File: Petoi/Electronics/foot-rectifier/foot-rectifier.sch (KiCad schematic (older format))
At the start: 6 parts, among them J1 Conn_01x04_Male, J2 Conn_01x02_Male

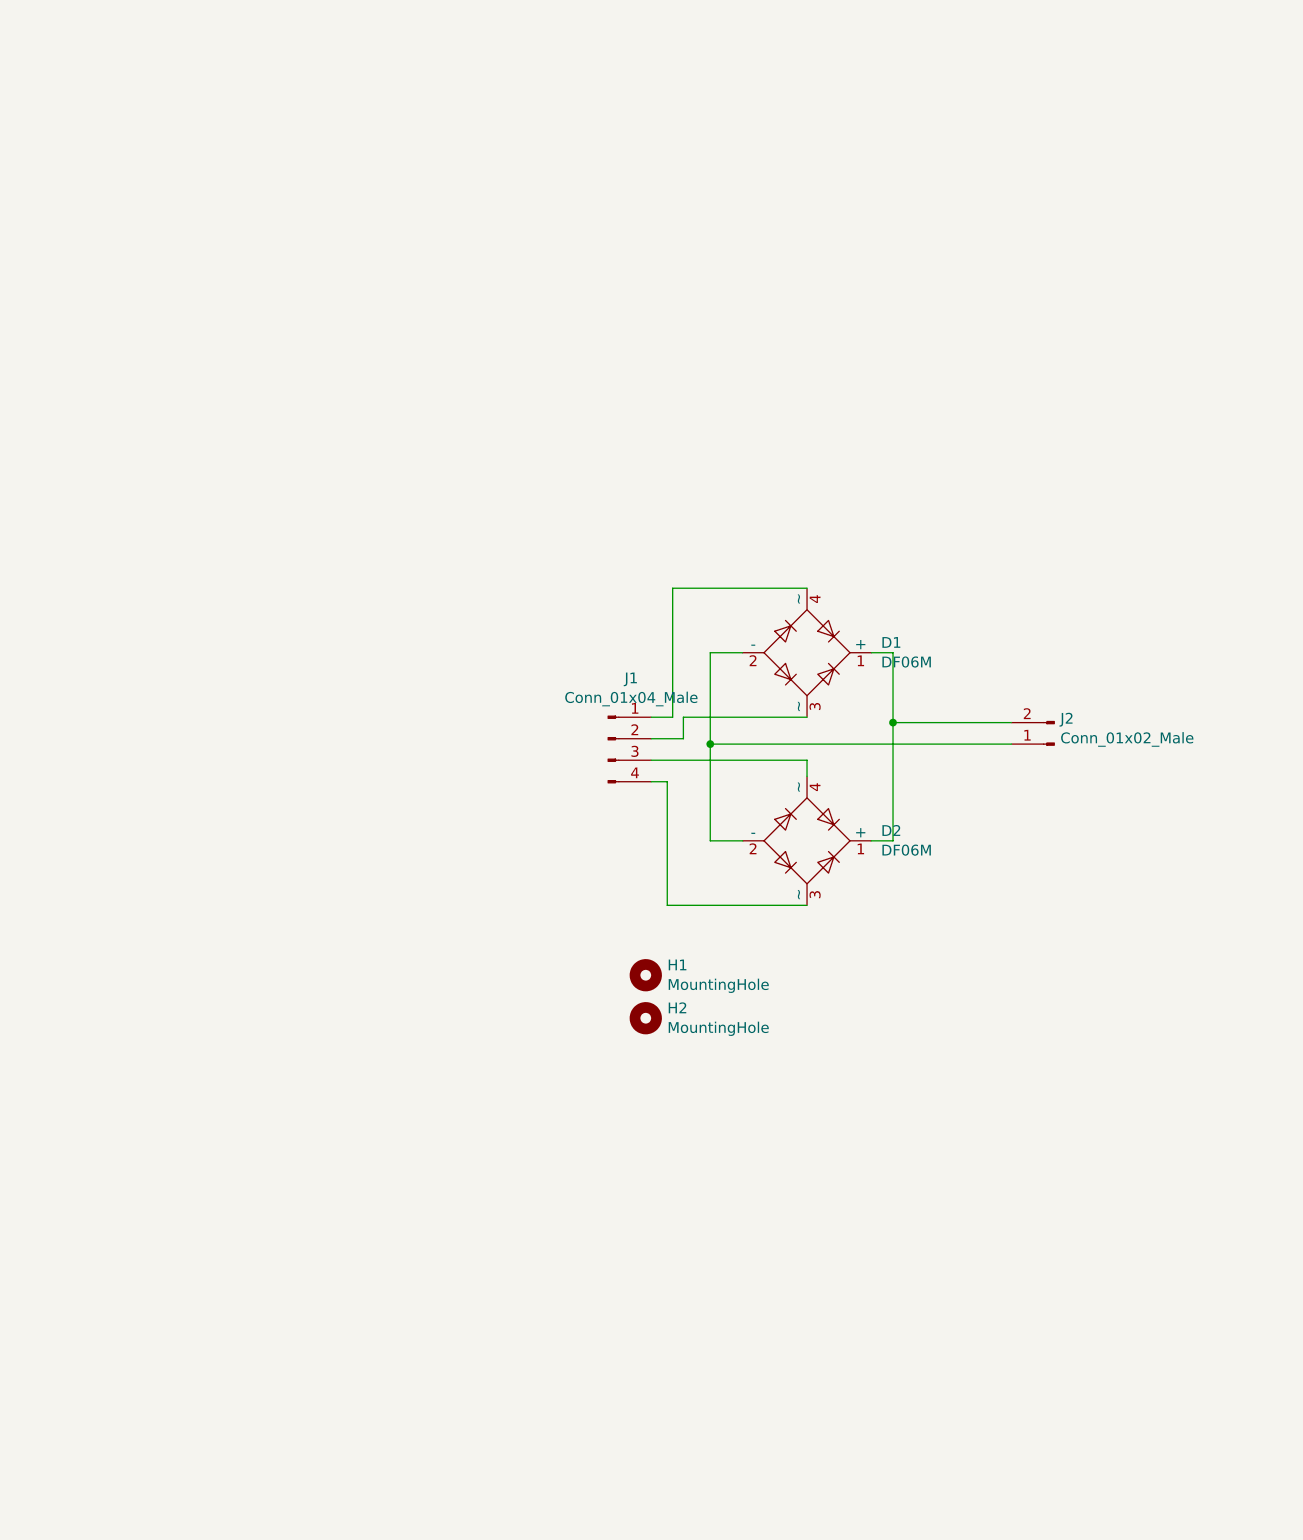
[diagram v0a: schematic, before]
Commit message: Sally's updated designs.
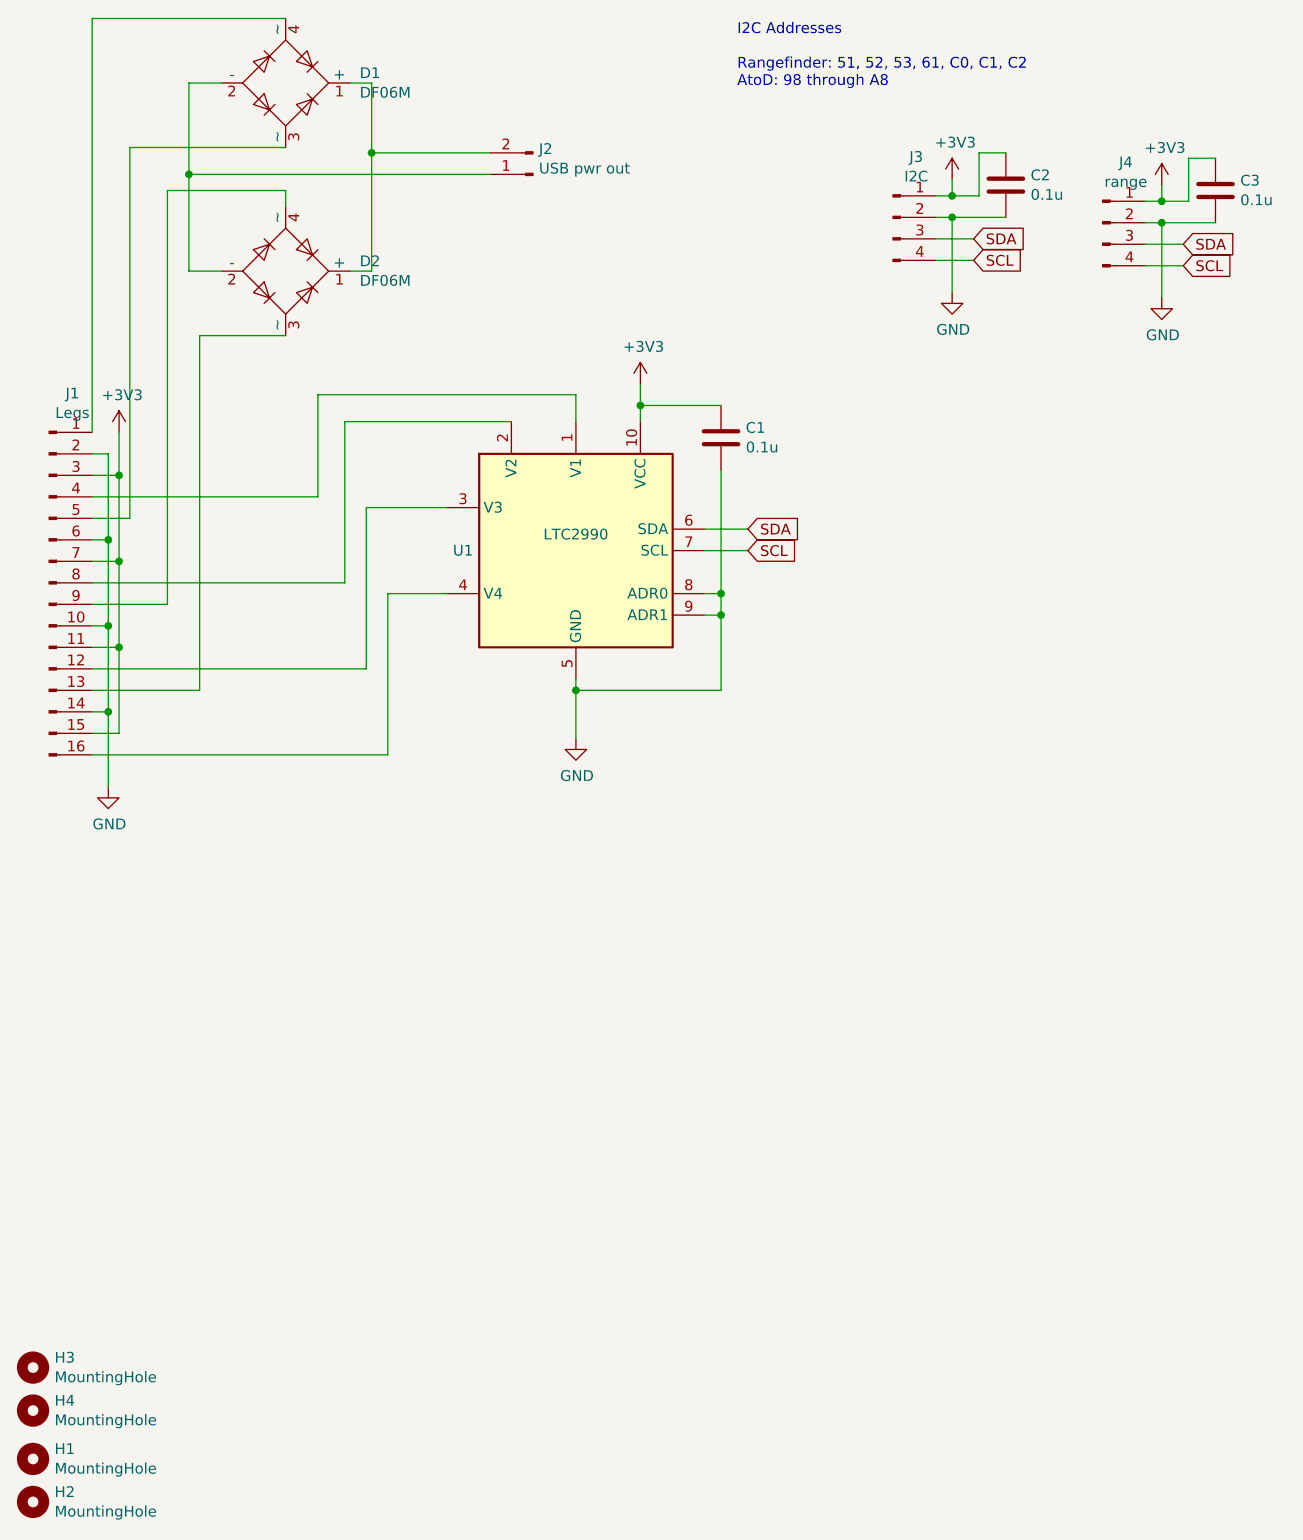
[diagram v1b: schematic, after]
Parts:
- removed J1: Conn_01x04_Male, Connector_PinHeader_2.54mm:PinHeader_1x04_P2.54mm_Vertical, symbol Connector:Conn_01x04_Male
- added C1, C2, C3: 0.1u, Capacitor_SMD:C_0805_2012Metric, symbol Device:C
- added H3, H4: MountingHole, MountingHole:MountingHole_2.5mm, symbol Mechanical:MountingHole
- added J1: Legs, Connector_PinSocket_2.54mm:PinSocket_1x16_P2.54mm_Vertical, symbol Connector:Conn_01x16_Male
- added J3: I2C, Connector_PinSocket_2.54mm:PinSocket_1x04_P2.54mm_Vertical, symbol Connector:Conn_01x04_Male
- added J4: range, Connector_PinSocket_2.54mm:PinSocket_1x04_P2.54mm_Vertical, symbol Connector:Conn_01x04_Male
- added U1: LTC2990, Package_SO:MSOP-10_3x3mm_P0.5mm, symbol Sensor:LTC2990
- J2: value Conn_01x02_Male -> USB pwr out
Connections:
- net at D1.3 (~~): now also J1.5 (Pin_5)
- net at D1.4 (~~): now also J1.1 (Pin_1)
- net at D2.3 (~~): now also J1.13 (Pin_13)
- net at D2.4 (~~): now also J1.9 (Pin_9)
- new net: J1.4 (Pin_4), U1.1 (V1)
- new net: J1.8 (Pin_8), U1.2 (V2)
- new net: J1.12 (Pin_12), U1.3 (V3)
- new net: J1.16 (Pin_16), U1.4 (V4)
- new net +3V3: C1.1, C2.1, C3.1, J1.11 (Pin_11), J1.15 (Pin_15), J1.3 (Pin_3), J1.7 (Pin_7), J3.1 (Pin_1), J4.1 (Pin_1), U1.10 (VCC)
- new net GND: C1.2, C2.2, C3.2, J1.10 (Pin_10), J1.14 (Pin_14), J1.2 (Pin_2), J1.6 (Pin_6), J3.2 (Pin_2), J4.2 (Pin_2), U1.5 (GND), U1.8 (ADR0), U1.9 (ADR1)
- new net SCL: J3.4 (Pin_4), J4.4 (Pin_4), U1.7 (SCL)
- new net SDA: J3.3 (Pin_3), J4.3 (Pin_3), U1.6 (SDA)
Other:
- note added: "I2C Addresses\n\nRangefinder: 51, 52, 53, 61, C0, C1, C2\nAtoD: 98 through A8"
- moved on the sheet: D1, D2, H1, H2, J2
